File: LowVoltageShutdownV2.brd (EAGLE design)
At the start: 23.8 x 21 mm, 7 parts

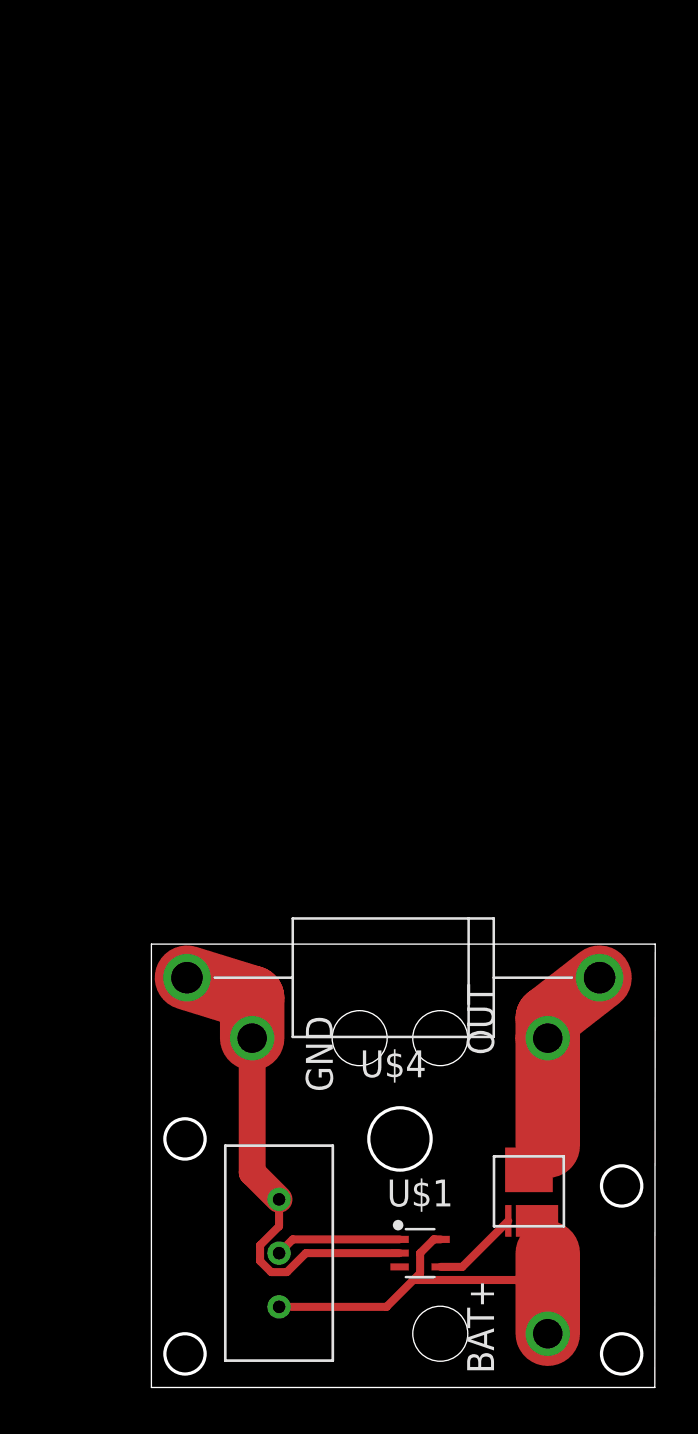
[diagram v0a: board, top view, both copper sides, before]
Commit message: second revision and added 3D models
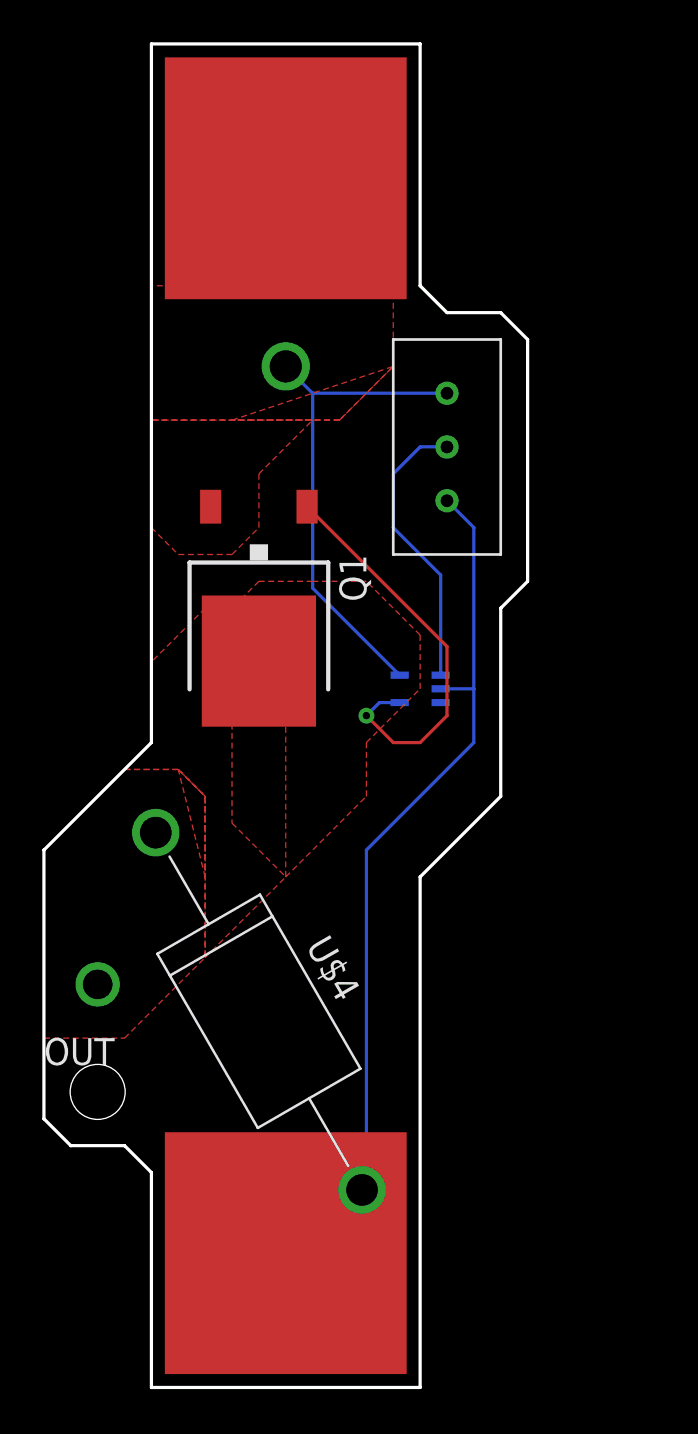
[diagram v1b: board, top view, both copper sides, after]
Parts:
- removed BAT+, GND: 16G, Wire2Board:16G
- removed U$2: SISS23DN-T1-GE3CY-ND, SISS23DN-T1-GE3CT-ND:POWERPAK1212-8S
- added Q1: FDD4141TO252, transistor-fet:TO252
- added U$5, U$6: 450PAD, Wire2Board:450PAD
- moved U$3 38.9 mm to (14.0, 44.5), turned to 180 degrees
- moved U$1 26.7 mm to (12.7, 33.0), flipped to the bottom
- moved OUT 21.4 mm to (-2.54, 19.1), turned to 270 degrees
- moved U$4 6.55 mm to (5.08, 17.8), turned to 300 degrees
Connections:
- removed net BAT+: BAT+.P$1, U$1.5, U$2.S, U$3.P$1
- new net BAT: Q1.2, U$1.5, U$3.P$1, U$5.P$1
- net GND: now also U$6.P$1; no longer GND.P$1
- net N$5: now also Q1.1; no longer U$2.G
- net OUT: now also Q1.3; no longer U$2.D
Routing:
- net BAT: track 0.00 -> 23.2 mm, vias 0 -> 1
- net BAT+: track 21.4 -> 0.00 mm
- net N$5: track 4.10 -> 19.3 mm, vias 0 -> 1
- net GND: track 23.7 -> 36.9 mm
- net OUT: track 10.6 -> 0.00 mm
- net N$1: track 5.97 -> 13.5 mm
- added copper zone on layer 1, net BAT
- added copper zone on layer 1, net OUT
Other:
- board size 23.8 x 21 mm -> 22.9 x 63.5 mm
